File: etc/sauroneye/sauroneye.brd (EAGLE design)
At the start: 70.8 x 57.1 mm, 9 parts, among them X1 USBSMD

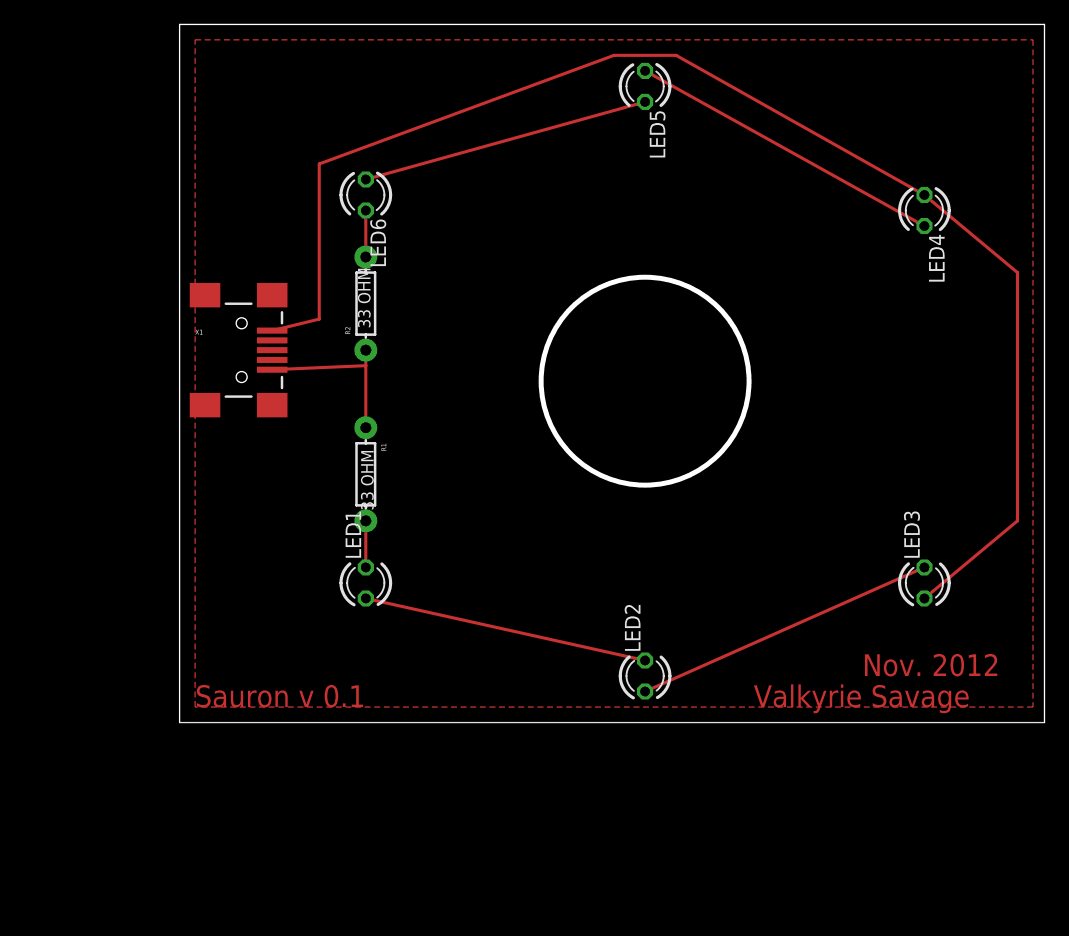
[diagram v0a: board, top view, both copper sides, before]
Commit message: new design files from Mark Oehlberg
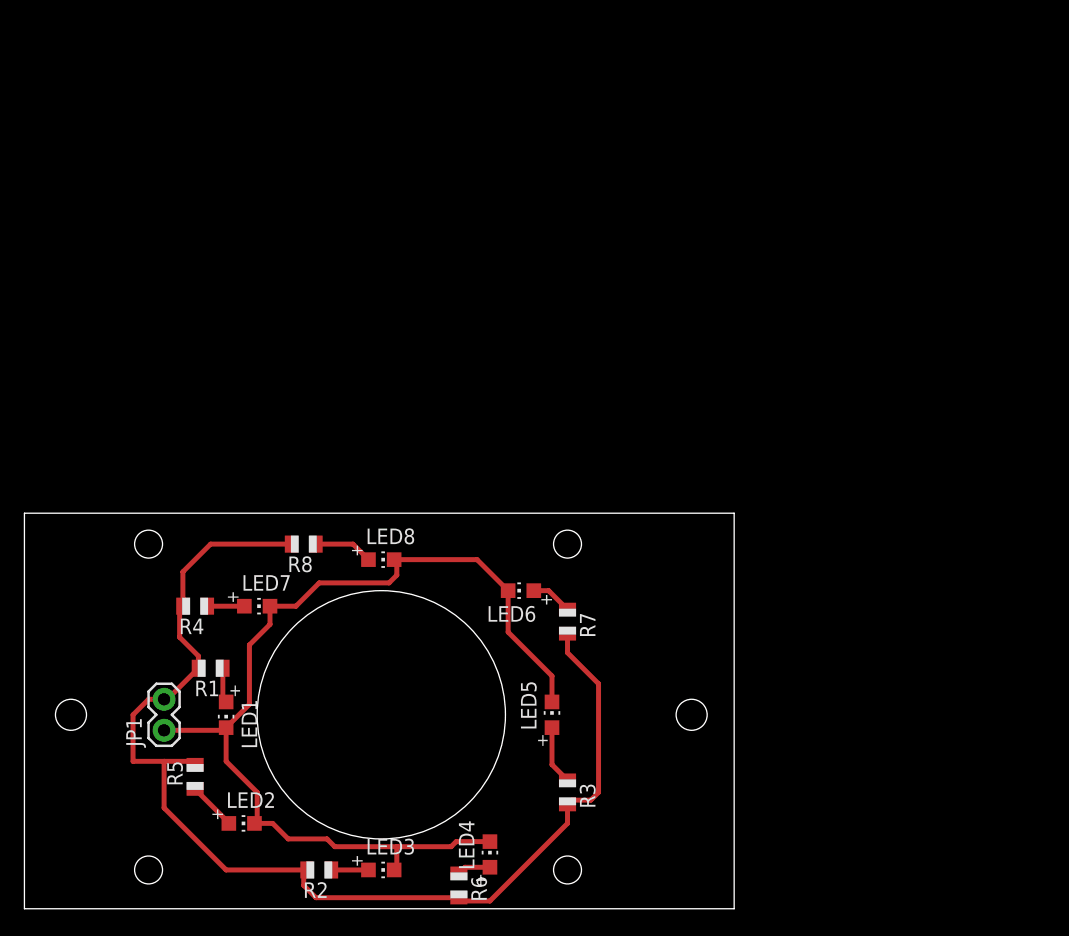
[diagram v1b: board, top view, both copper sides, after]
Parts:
- removed X1: USBSMD, SparkFun:USB-MINIB
- added JP1: (no value), SparkFun-Connectors:1X02
- added LED7, LED8: (no value), adafruit:CHIP-LED0805
- added R3, R4, R5, R6, R7, R8: 100, adafruit:R0805
- LED1, LED2, LED3, LED4, LED5, LED6: value TLLG4400 -> (none); device led:LED3MM -> adafruit:CHIP-LED0805
- R1, R2: value 33 OHM -> 100; device SparkFun:AXIAL-0.3 -> adafruit:R0805
- moved LED4 63.6 mm to (38.1, 4.45), turned to 0 degrees
- moved LED5 52.0 mm to (43.2, 15.9), turned to 0 degrees
- moved LED3 50.3 mm to (29.2, 3.17), turned to 270 degrees
- moved R2 46.5 mm to (24.1, 3.17), turned to 180 degrees
- moved LED2 35.2 mm to (17.8, 6.99), turned to 270 degrees
- moved LED6 34.8 mm to (40.6, 26.0), turned to 90 degrees
- moved R1 20.3 mm to (15.2, 19.7), turned to 180 degrees
- moved LED1 15.7 mm to (16.5, 15.9), turned to 180 degrees
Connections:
- removed net GND: R1.P$1, R2.P$1, X1.GND
- removed net VCC: LED3.A, LED4.A, X1.VBUS
- new net N$10: LED8.A, R8.1
- new net N$7: LED2.A, R5.1
- new net N$8: LED4.A, R6.1
- new net N$9: LED6.A, R7.1
- net N$1: now also JP1.2, R1.2, R2.2, R3.2, R4.2, R5.2, R6.2, R7.2, R8.2; no longer LED6.K, R2.P$2
- net N$2: now also LED1.A, R1.1; no longer LED1.K, R1.P$2
- net N$3: now also LED3.A, R2.1; no longer LED5.K, LED6.A
- net N$4: now also R3.1; no longer LED4.K
- net N$5: now also LED7.A, R4.1; no longer LED1.A, LED2.K
- net N$6: now also JP1.1, LED1.C, LED2.C, LED3.C, LED4.C, LED5.C, LED6.C, LED7.C, LED8.C; no longer LED2.A, LED3.K
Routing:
- net VCC: track 110.9 -> 0.00 mm
- net N$1: track 3.81 -> 96.7 mm
- net N$6: track 25.0 -> 81.6 mm
- net N$4: track 26.2 -> 4.83 mm
- net N$3: track 23.7 -> 3.03 mm
- net N$5: track 23.4 -> 3.03 mm
- net GND: track 14.0 -> 0.00 mm
- net N$10: track 0.00 -> 4.83 mm
- net N$7: track 0.00 -> 3.95 mm
- net N$9: track 0.00 -> 3.40 mm
- net N$8: track 0.00 -> 2.74 mm
- net N$2: track 3.81 -> 2.87 mm
- removed copper zone on layer 1, net GND
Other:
- board size 70.8 x 57.1 mm -> 58.1 x 32.4 mm
- board text removed: "Nov. 2012"
- board text removed: "Sauron v 0.1"
- board text removed: "Valkyrie Savage"
